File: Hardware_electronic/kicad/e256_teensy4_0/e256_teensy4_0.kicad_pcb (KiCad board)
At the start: 2 copper layers, 76 x 70 mm, 58 parts, among them J0 Conn_Coaxial_Power, J1 MIDI_IN, J2 MIDI_OUT, J3 AUDIO_IN, J4 AUDIO_OUT, J5 LINE_OUT, J6 e256_pad_16x16, SW1 SW_Push, SW2 SW_Push, SW3 RotaryEncoder_Switch, U1 6N138SM, U10 W25Q128JVS, U2 Teensy4.0, U3 74HC595BQ, U4 74HC595BQ, U5 74HC595BQ, U6 74HC4051BQ, U7 74HC4051BQ, U8 MCP1811A, U9 SGTL5000

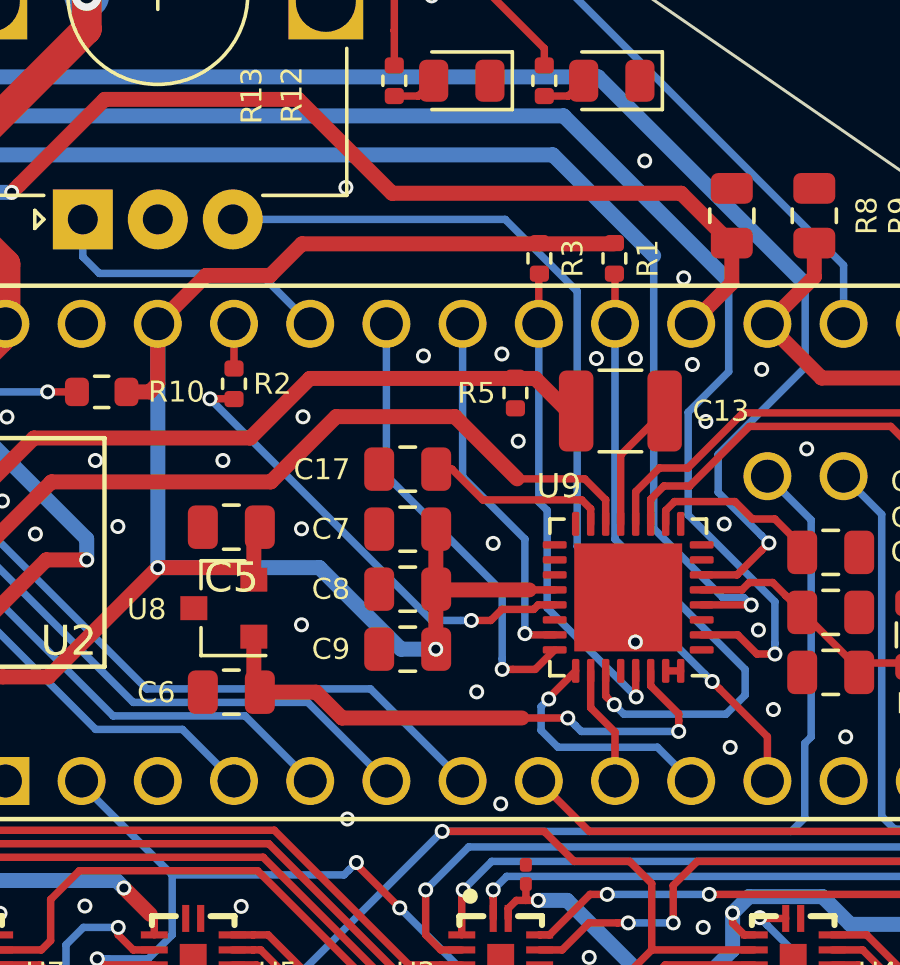
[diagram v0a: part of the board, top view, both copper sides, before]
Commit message: Minor Changes & update README
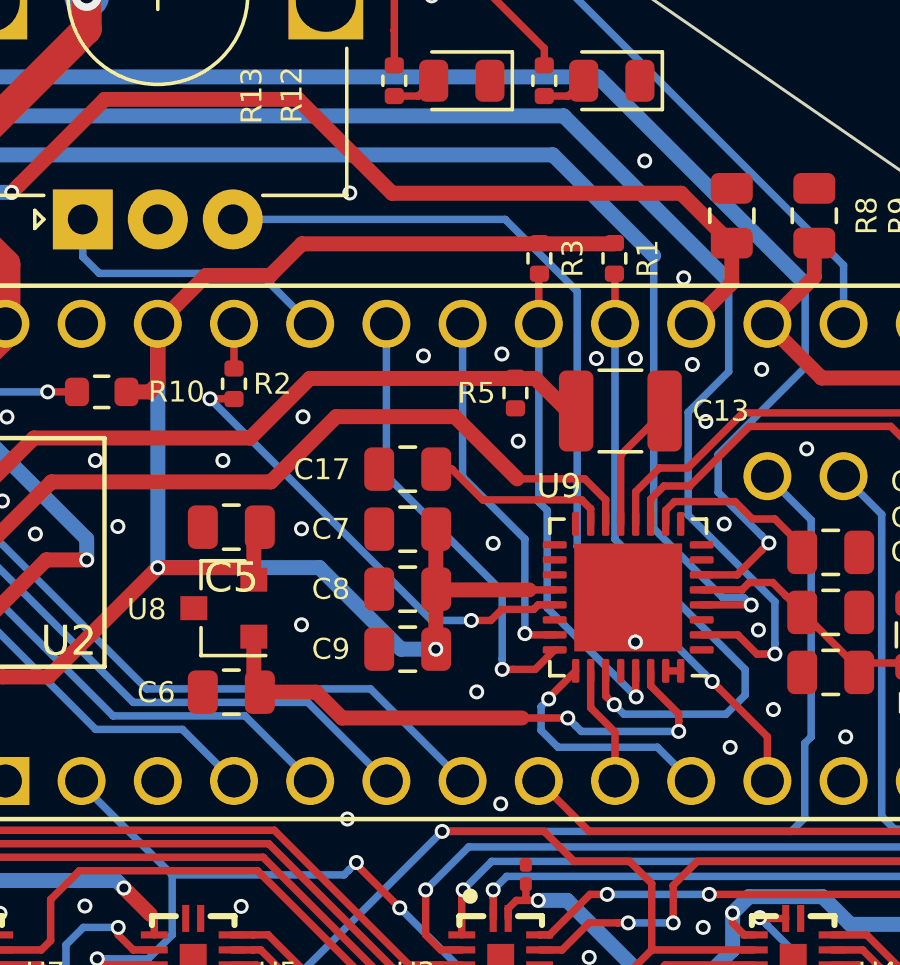
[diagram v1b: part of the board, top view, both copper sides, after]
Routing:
- net MEM_CS: track 23.1 -> 22.5 mm
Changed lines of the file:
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@@
     (thickness 1.2)
     (drawings 627)
-    (tracks 998)
+    (tracks 997)
     (zones 0)
     (modules 58)
@@
   (via (at 151.26 111.758) (size 0.5) (drill 0.3) (layers F.Cu B.Cu) (net 28))
   (via (at 146.51 75.908) (size 0.5) (drill 0.3) (layers F.Cu B.Cu) (net 28))
-  (via (at 143.649949 82.29494) (size 0.5) (drill 0.3) (layers F.Cu B.Cu) (net 28))
+  (via (at 143.779949 82.47694) (size 0.5) (drill 0.3) (layers F.Cu B.Cu) (net 28))
   (via (at 153.61 81.408) (size 0.5) (drill 0.3) (layers F.Cu B.Cu) (net 28))
   (via (at 154.91 85.308) (size 0.5) (drill 0.3) (layers F.Cu B.Cu) (net 28))
@@
   (segment (start 169.449949 93.944934) (end 164.117943 99.27694) (width 0.25) (layer B.Cu) (net 67))
   (via (at 164.079949 99.27694) (size 0.5) (drill 0.3) (layers F.Cu B.Cu) (net 67))
-  (segment (start 150.08 102.078) (end 150.715 102.078) (width 0.25) (layer F.Cu) (net 68))
   (segment (start 165.47 97.993) (end 165.655 97.808) (width 0.25) (layer F.Cu) (net 68))
   (segment (start 164.06 97.993) (end 165.47 97.993) (width 0.25) (layer F.Cu) (net 68))
